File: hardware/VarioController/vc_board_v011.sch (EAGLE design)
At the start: 32 parts, among them IC1 WeMos D1 mini, K1 AQY21SOP, K2 AQY21SOP, K3 AQY21SOP, K4 AQY21SOP, X2 SPTAF_1/8_3,5, X3 05-JST-B5B-XH-A, X4 SPTAF_1/8_3,5

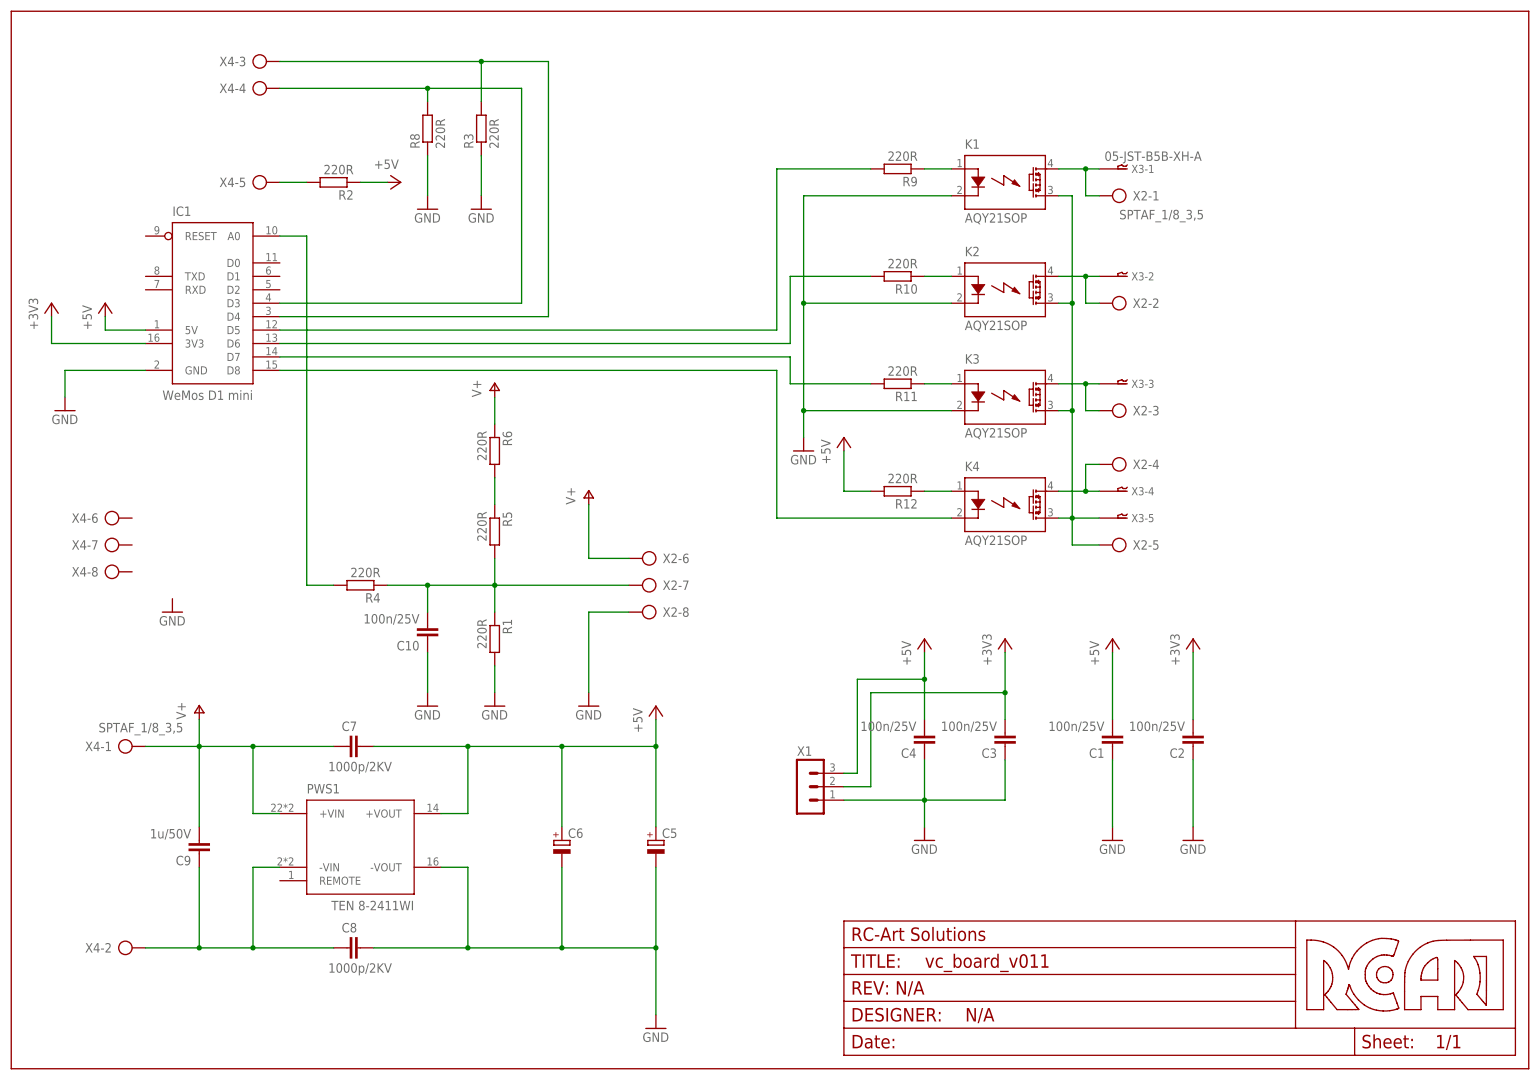
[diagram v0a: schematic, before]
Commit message: Add layout
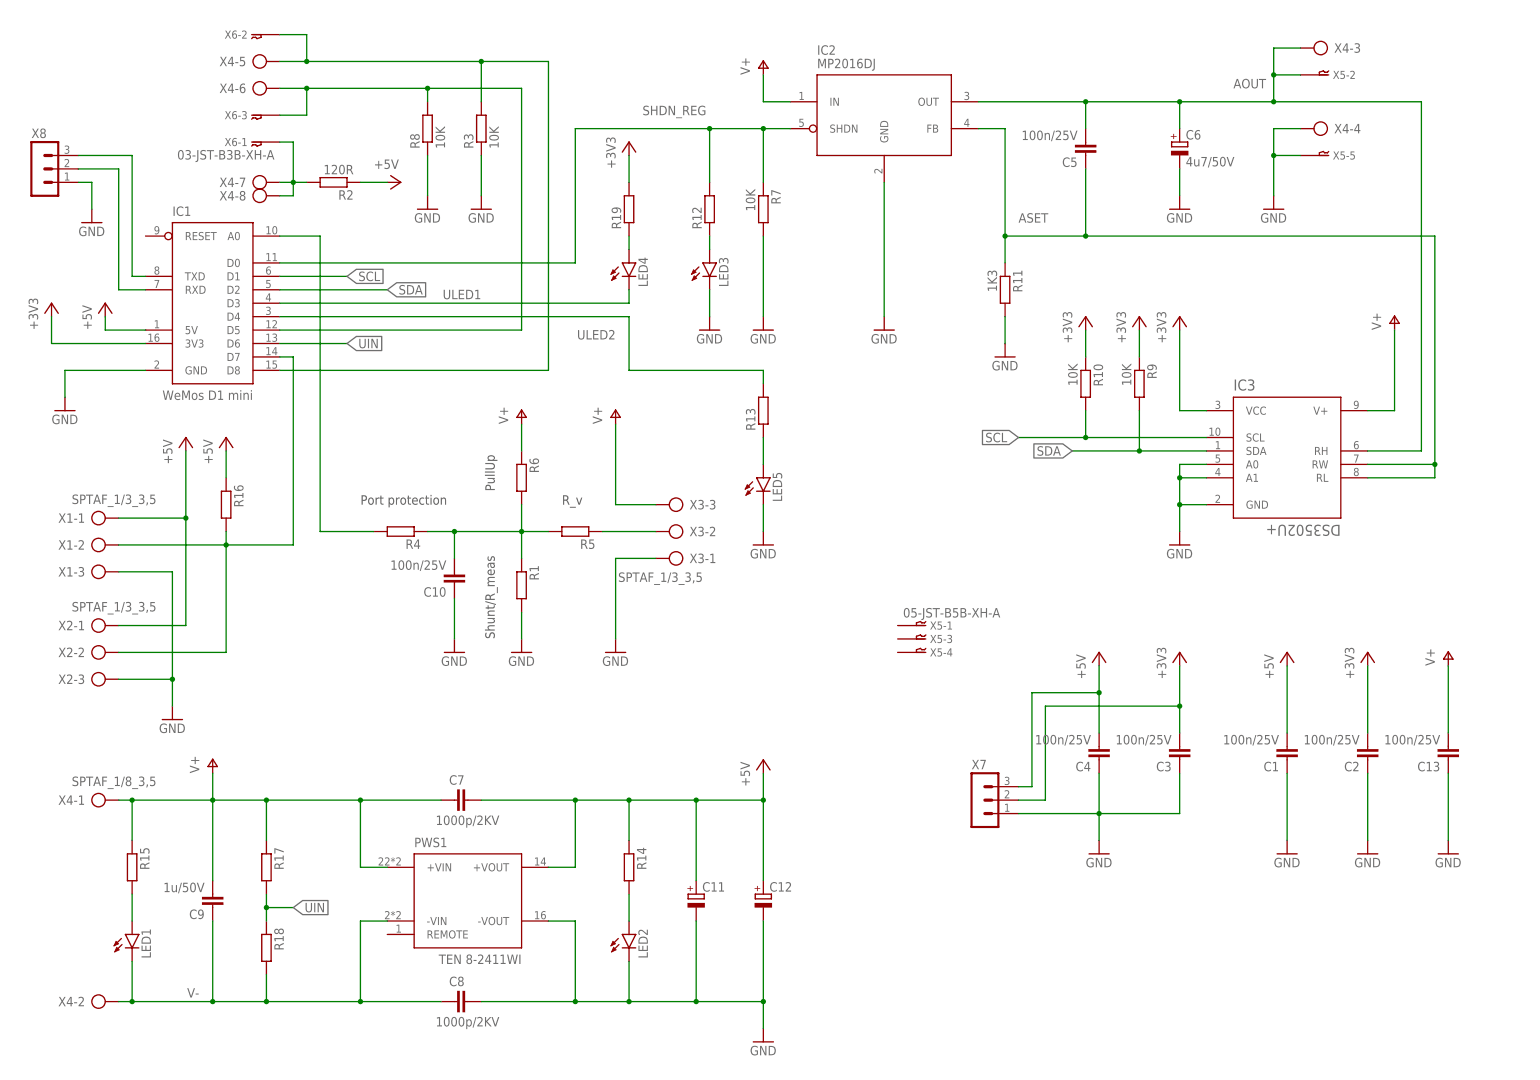
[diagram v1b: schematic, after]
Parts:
- removed FRAME1: MF_FRAMEDEFAULT, rca-frames:MF_FRAMEDEFAULT
- removed K1, K2, K3, K4: AQY21SOP, relay:AQY21SOP
- added C11, C12: (no value), rcl:CPOL-EUD/7343-31W
- added C13: 100n/25V, rcl:C-EUC0805
- added IC2: MP2016DJ, mps-regulator:MP2016
- added IC3: DS3502U+, maxim-ds3502:DS3502U+
- added LED1, LED2, LED3, LED4, LED5: (no value), led:LEDCHIPLED_0805
- added R13, R14, R15, R16, R17, R18, R19: (no value), rcl:R-EU_R0805
- added R7: 10K, rcl:R-EU_R0805
- added X5: 05-JST-B5B-XH-A, con-jst-xh:05-JST-B5B-XH-A
- added X6: 03-JST-B3B-XH-A, con-jst-xh:03-JST-B3B-XH-A
- added X7, X8: (no value), con-lstb:MA03-1
- C5: value (none) -> 100n/25V; device rcl:CPOL-EUCT7343 -> rcl:C-EUC0805
- C6: value (none) -> 4u7/50V; device rcl:CPOL-EUCT7343 -> rcl:CPOL-EUD/7343-31W
- R1, R12, R4, R5, R6: value 220R -> (none)
- R10, R3, R8, R9: value 220R -> 10K
- R11: value 220R -> 1K3
- R2: value 220R -> 120R
- X1: value (none) -> SPTAF_1/3_3,5; device con-lstb:MA03-1 -> con-phoenix-sptaf:SPTAF_1/3_3,5
- X2: value SPTAF_1/8_3,5 -> SPTAF_1/3_3,5; device con-phoenix-sptaf:SPTAF_1/8_3,5 -> con-phoenix-sptaf:SPTAF_1/3_3,5
- X3: value 05-JST-B5B-XH-A -> SPTAF_1/3_3,5; device con-jst-xh:05-JST-B5B-XH-A -> con-phoenix-sptaf:SPTAF_1/3_3,5
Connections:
- removed net N$11: K4.A, R12.1
- removed net N$12: R5.1, R6.2
- removed net N$20: IC1.D5, R9.2
- removed net N$4: C8.1, C9.1, PWS1.-VIN, X4-2.KL
- removed net N$7: K4.DS1, X2-4.KL, X3-4.1
- removed net N$8: K3.DS1, X2-3.KL, X3-3.1
- removed net N$9: K2.DS1, X2-2.KL, X3-2.1
- new net AOUT: C5.2, C6.+, IC2.OUT, IC3.RH, X4-3.KL, X5-2.1
- new net ASET: C5.1, IC2.FB, IC3.RL, IC3.RW, R11.1
- new net N$15: IC1.D7, R16.2, X1-2.KL, X2-2.KL
- new net SCL: IC1.D1, IC3.SCL, R10.2
- new net SDA: IC1.D2, IC3.SDA, R9.2
- new net SHDN_REG: IC1.D0, IC2.SHDN, R12.2, R7.1
- new net UIN: IC1.D6, R17.2, R18.1
- new net ULED1: IC1.D3, LED4.C
- new net ULED2: IC1.D4, R13.2
- new net V-: C8.1, C9.1, LED1.C, PWS1.-VIN, R18.2, X4-2.KL
- net +3V3: now also IC3.VCC, R10.1, R19.2, R9.1, X7.2; no longer X1.2
- net +5V: now also C11.+, C12.+, R14.1, R16.1, X1-1.KL, X2-1.KL, X7.3; no longer C5.+, C6.+, R12.2, X1.3
- net GND: now also C11.-, C12.-, C13.1, IC2.GND, IC3.A0, IC3.A1, IC3.GND, LED2.C, LED3.C, LED5.C, R11.2, R7.2, X1-3.KL, X2-3.KL, X3-1.KL, X4-4.KL, X5-5.1, X7.1, X8.1; no longer C5.-, K1.K, K2.K, K3.K, X1.1, X2-8.KL
- net N$1: now also R6.2; no longer X2-7.KL
- net N$10: now also LED3.A, R12.1; no longer K1.DS1, X2-1.KL, X3-1.1
- net N$13: now also LED1.A, R15.2; no longer K3.A, R11.1
- net N$14: now also LED2.A, R14.2; no longer K2.A, R10.1
- net N$16: now also IC1.TXD, X8.3; no longer K1.A, R9.1
- net N$17: now also IC1.RXD, X8.2; no longer IC1.D8, K4.K
- net N$18: now also LED4.A, R19.1; no longer IC1.D7, R11.2
- net N$19: now also LED5.A, R13.1; no longer IC1.D6, R10.2
- net N$2: now also IC1.D5, X4-6.KL, X6-3.1; no longer IC1.D3, X4-4.KL
- net N$3: now also IC1.D8, X4-5.KL, X6-2.1; no longer IC1.D4, X4-3.KL
- net N$5: now also X4-7.KL, X4-8.KL, X6-1.1; no longer X4-5.KL
- net N$6: now also R5.1, X3-2.KL; no longer K1.DS2, K2.DS2, K3.DS2, K4.DS2, X2-5.KL, X3-5.1
- net V+: now also C13.2, IC2.IN, IC3.V+, R15.1, R17.1, X3-3.KL; no longer X2-6.KL
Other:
- note added: "Port protection"
- note added: "PullUp"
- note added: "R_v"
- note added: "Shunt/R_meas"
- moved on the sheet: C1, C10, C2, C3, C4, C6, C7, C8, C9, PWS1, R1, R10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
